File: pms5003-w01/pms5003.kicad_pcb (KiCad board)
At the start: 2 copper layers, 60 x 56 mm, 28 parts, among them J1 Battery, J2 DS3231, J3 PMS5003, J4 SHT10, J5 P2, J6 PROG, J7 USB_OTG, Q1 IRF540N, Q2 IRF7309IPBF, U1 U3V12F5, U11 W01, U2 MAX1811, U3 TC1262-33

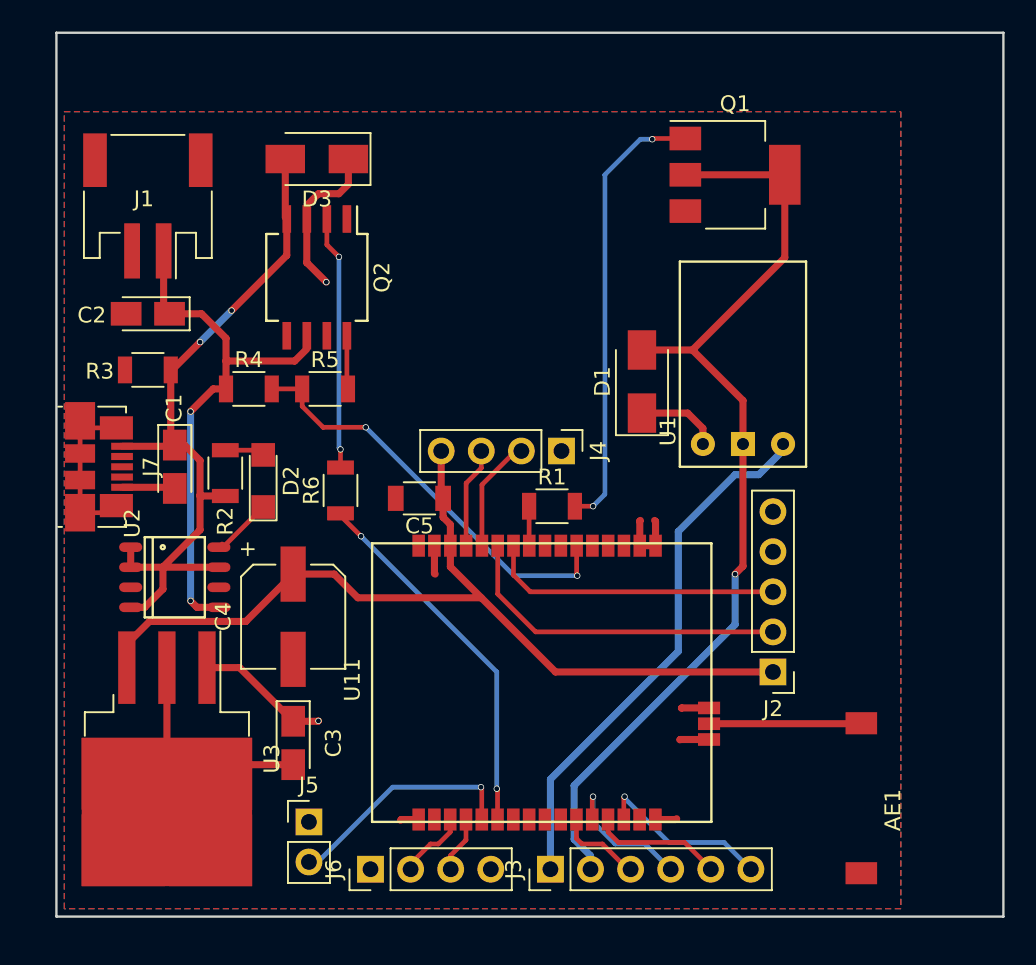
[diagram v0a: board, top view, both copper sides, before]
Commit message: Next iteration of w01 pms5003
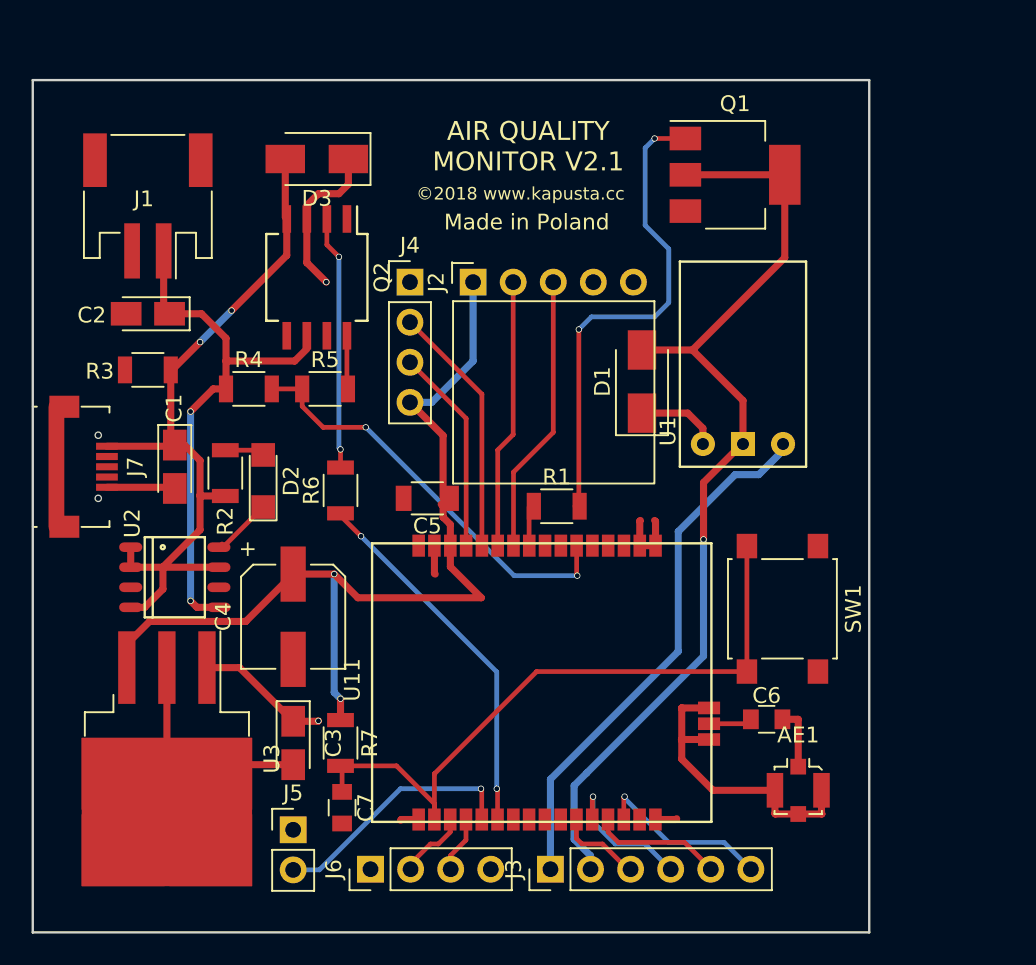
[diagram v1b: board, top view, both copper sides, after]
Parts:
- added C6: 22pF, Capacitors_SMD:C_0805, F.Cu at (166.0, 68.5)
- added C7: 1nF, Capacitors_SMD:C_0805, F.Cu at (139.1, 74.1)
- added R7: 10k, Resistors_SMD:R_1206, F.Cu at (139.0, 70.0)
- added SW1: SW_Push, Buttons_Switches_SMD:SW_SPST_B3S-1000, F.Cu at (167.0, 61.5)
- AE1: value Antenna -> Antenna_Shield; footprint various:Rainsun_AN9520 -> Connector_Coaxial:U.FL_Molex_MCRF_73412-0110_Vertical
- J2: footprint Socket_Strips:Socket_Strip_Straight_1x05_Pitch2.54mm -> various:DS3231
- J5: footprint Socket_Strips:Socket_Strip_Straight_1x02_Pitch2.54mm -> Pin_Headers:Pin_Header_Straight_1x02_Pitch2.54mm
- J7: footprint Connectors_USB:USB_Micro-B_Molex_47346-0001 -> various:USB_Micro-B_91-US01-517
- R2: value 100 -> 470
- moved J2 31.2 mm to (147.4, 40.8), turned to 90 degrees
- moved J4 14.4 mm to (143.4, 40.8), turned to 0 degrees
- moved AE1 4.03 mm to (168.0, 73.0), turned to 180 degrees
- moved J5 1.12 mm to (136.0, 75.5)
- moved C5 0.50 mm to (144.5, 54.5)
- moved R1 0.30 mm to (152.7, 55.0)
- moved J7 0.20 mm to (122.7, 52.5)
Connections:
- AE1 pad 2: (no net) -> -USB
- U11 pad 16: Net-(AE1-Pad1) -> Net-(C6-Pad1)
- U11 pad 2: (no net) -> RST
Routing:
- net RST: track 0.00 -> 43.0 mm
- net -USB: track 34.0 -> 51.0 mm
- net SHT10_SCK: track 7.25 -> 16.0 mm
- net SHT10_DATA: track 6.40 -> 13.1 mm
- net Net-(AE1-Pad1): track 9.66 -> 4.00 mm
- net RTC_SDA: track 21.5 -> 17.1 mm
- net Net-(J7-Pad6): track 10.8 -> 7.60 mm
- net Net-(C6-Pad1): track 0.00 -> 2.77 mm
- net 3V3: track 57.2 -> 59.8 mm, vias 0 -> 2
- net Net-(Q1-Pad1): track 28.6 -> 31.0 mm
- net +USB: track 47.0 -> 48.2 mm
- net P2: track 14.9 -> 16.0 mm
- net RTC_SCL: track 18.7 -> 17.7 mm
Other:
- board size 60 x 56 mm -> 53 x 54 mm
- net class USBCON added: clearance 0.2, trace_width 1, via_dia 0.4, via_drill 0.3
- board text added: "AIR QUALITY MONITOR V2.1"
- board text added: "Made in Poland"
- board text added: "©2018 www.kapusta.cc"
